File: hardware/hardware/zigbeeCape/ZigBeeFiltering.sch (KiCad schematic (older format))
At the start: 35 parts, among them U3 SMA_Antenna

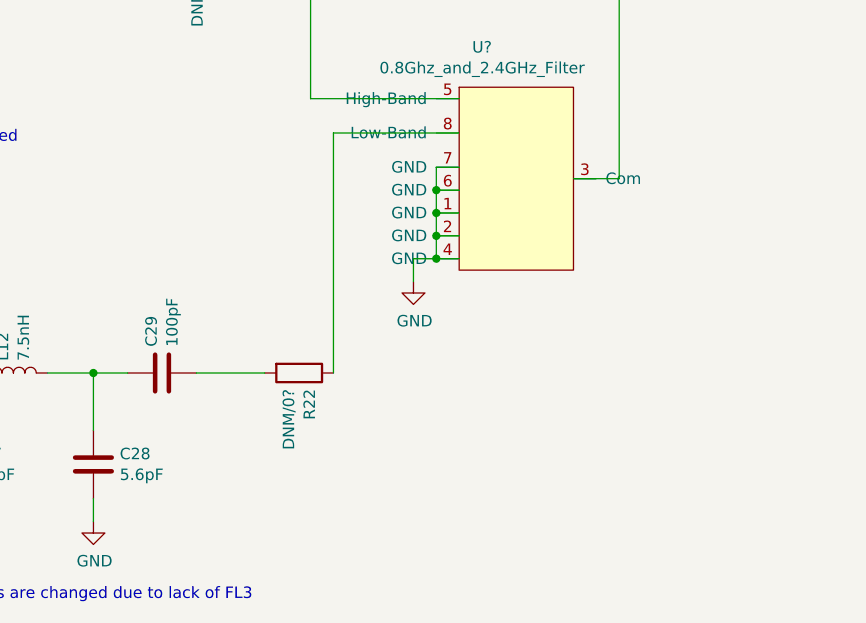
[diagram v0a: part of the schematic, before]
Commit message: Fixed a few little things
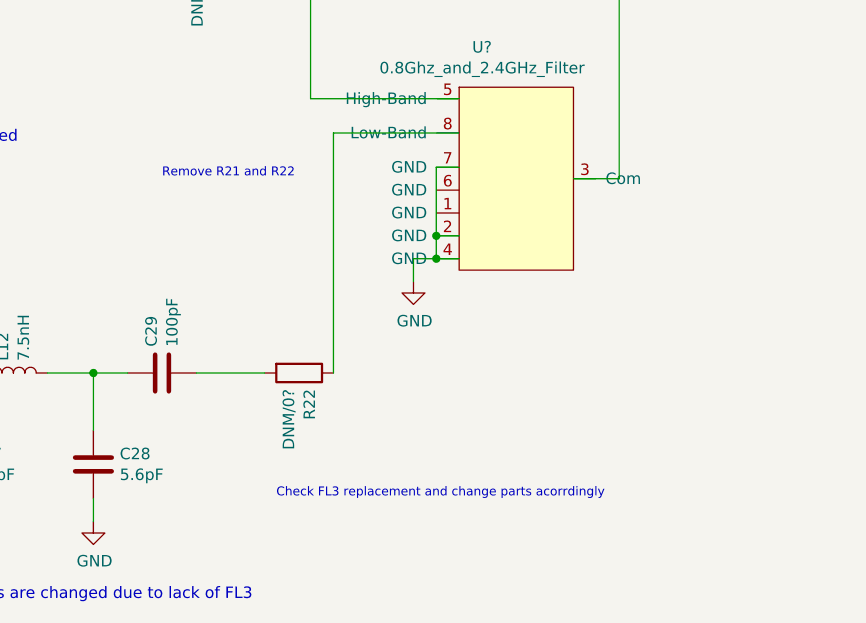
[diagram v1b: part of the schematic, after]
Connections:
- net GND: no longer U?.1 (GND), U?.6 (GND)
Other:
- note added: "Check FL3 replacement and change parts acorrdingly"
- note added: "Remove R21 and R22"
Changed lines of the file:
@@
 	6750 4250 6650 4250
-Wire Wire Line
-	6650 4250 6650 4350
-Wire Wire Line
-	6650 4350 6750 4350
-Wire Wire Line
-	6750 4450 6650 4450
 Wire Wire Line
 	6650 4550 6750 4550
 Wire Wire Line
 	6750 4650 6650 4650
-Wire Wire Line
-	6650 4350 6650 4450
-Connection ~ 6650 4350
-Connection ~ 6650 4450
-Wire Wire Line
-	6650 4450 6650 4550
 Connection ~ 6650 4550
 Wire Wire Line
@@
 	7450 4300 7250 4300
 Connection ~ 7450 3400
+Text Notes 5450 4300 0    39   ~ 0
+Remove R21 and R22
+Text Notes 5950 5700 0    39   ~ 0
+Check FL3 replacement and change parts acorrdingly
+Wire Wire Line
+	6650 4250 6650 4550
 $EndSCHEMATC

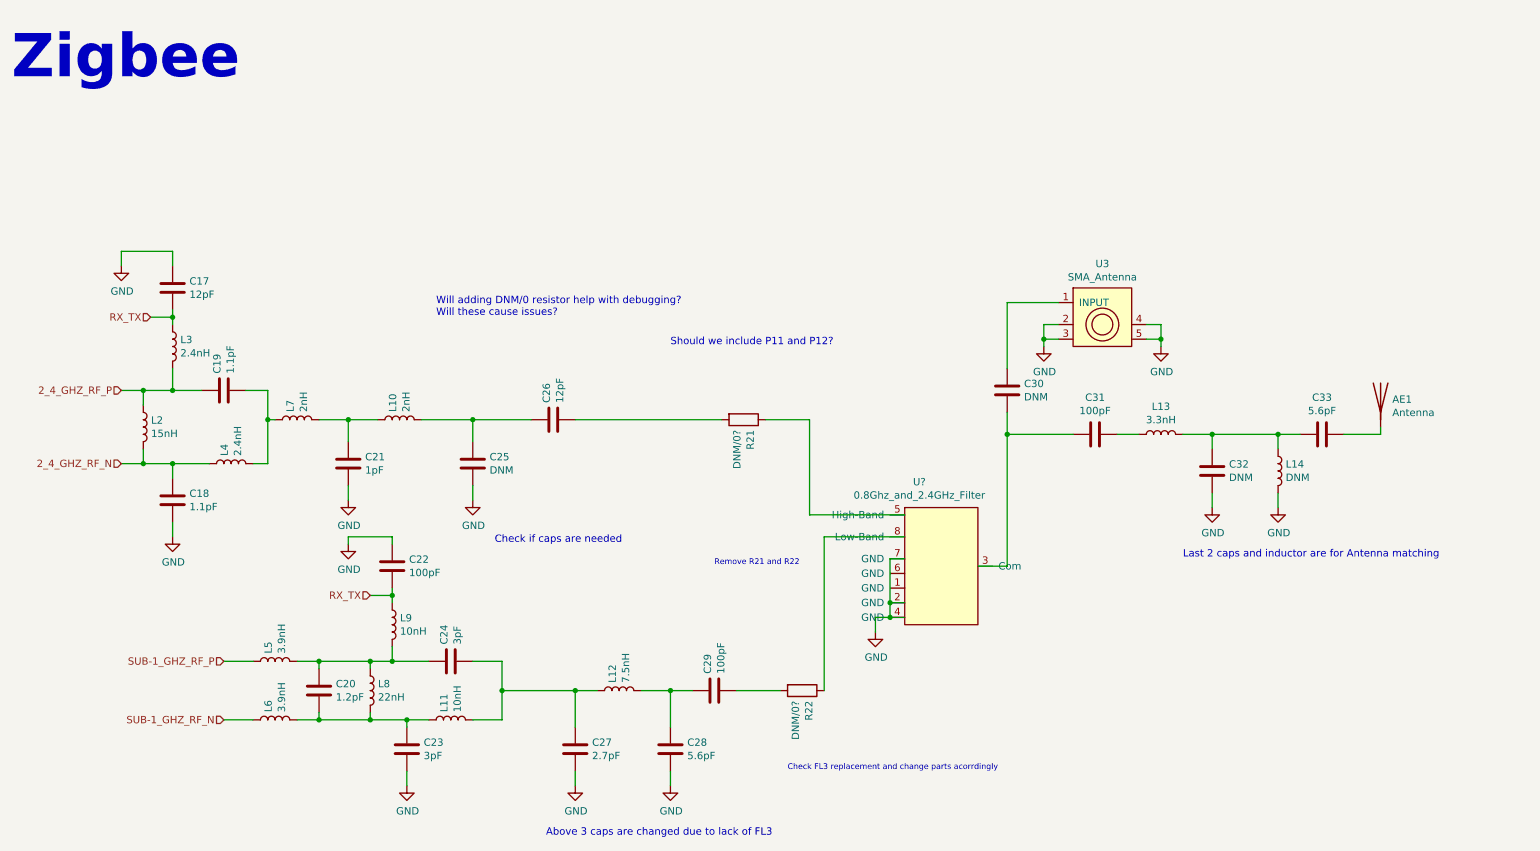
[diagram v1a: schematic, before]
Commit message: Fixing Git issue
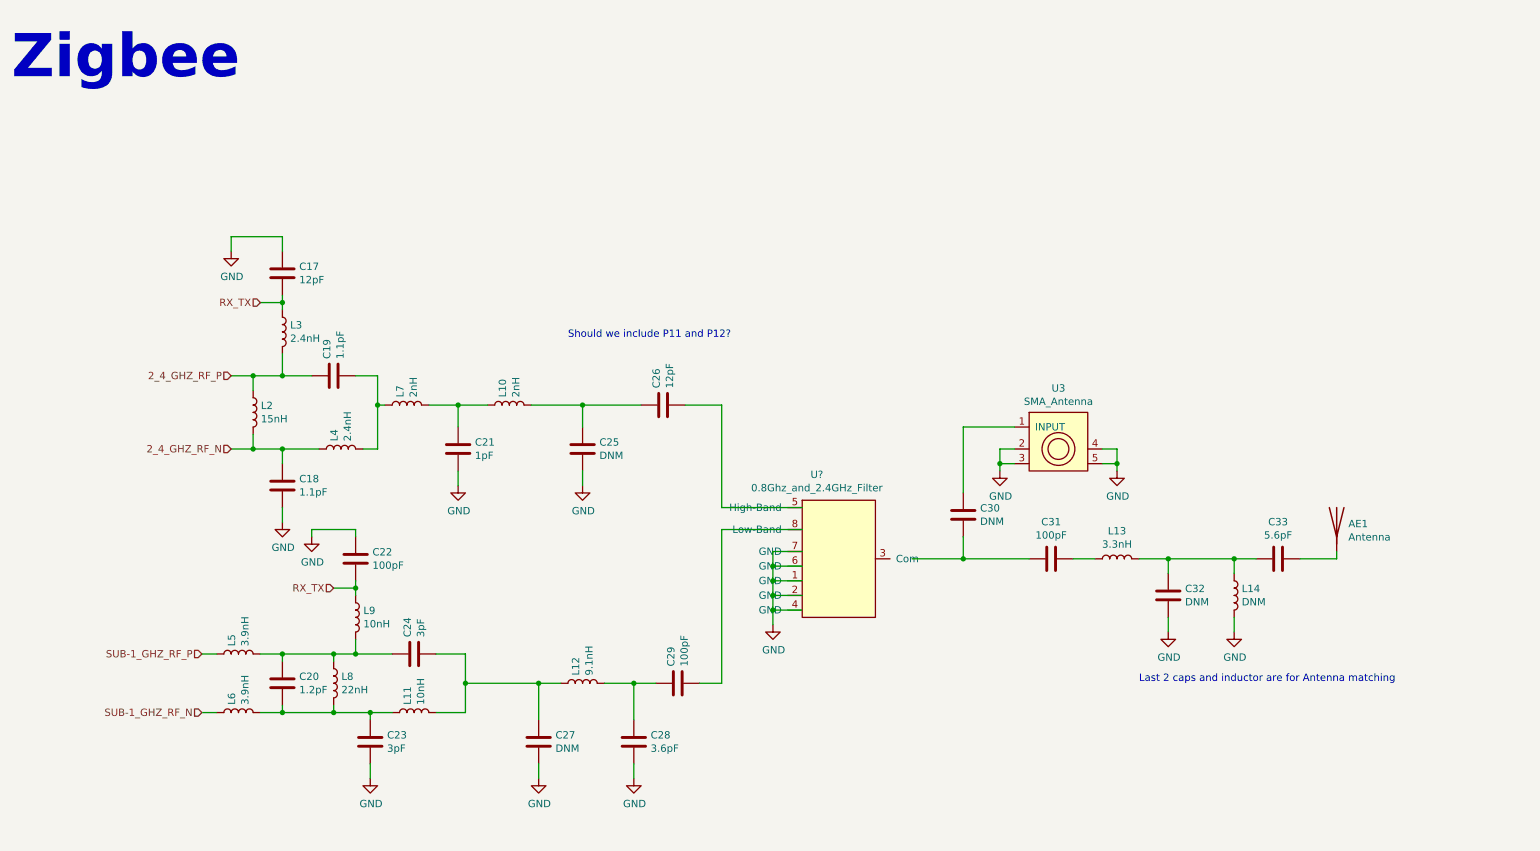
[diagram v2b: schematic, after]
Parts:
- removed R21, R22: DNM/0?, symbol Device:R
- C27: value 2.7pF -> DNM
- C28: value 5.6pF -> 3.6pF
- L12: value 7.5nH -> 9.1nH
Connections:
- net GND: now also U?.1 (GND), U?.6 (GND)
- net at C26.2: now also U?.5 (High-Band)
- net at C29.2: now also U?.8 (Low-Band)
- net at C30.2, C31.2: no longer U?.3 (Com)
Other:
- note removed: "Above 3 caps are changed due to lack of FL3"
- note removed: "Check FL3 replacement and change parts acorrdingly"
- note removed: "Check if caps are needed"
- note removed: "Remove R21 and R22"
- note removed: "Will adding DNM/0 resistor help with debugging?\nWill these cause issues?"
- moved on the sheet: AE1, C17, C18, C19, C20, C21, C22, C23, C24, C25, C26, C27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
